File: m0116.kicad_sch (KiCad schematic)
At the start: 256 parts, among them J2 Conn_01x04_MountingPin, J3 Conn_01x04_MountingPin, Q1 Q_PMOS_GSD AO3401A, Q2 Q_NMOS_GSD 2N7002, Q3 Q_NMOS_GSD 2N7002, Q4 2N3904, SW1 SW_Push, U1 XC6206P332MR, U2 74AHCT1G125, U3 STM32F411RETx, U4 24LC64, U5 USBLC6-2SC6, Y1 8MHz

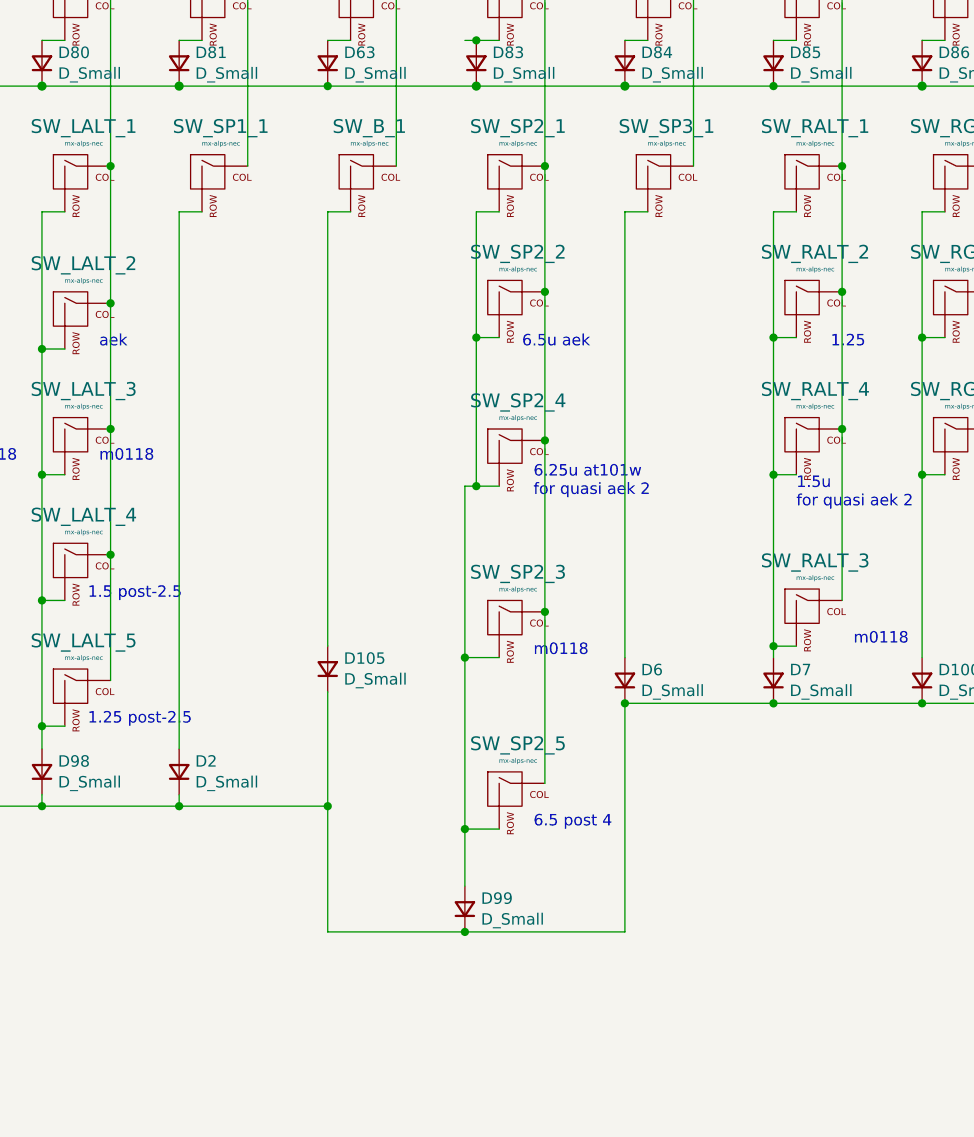
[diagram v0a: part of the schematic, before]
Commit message: fix
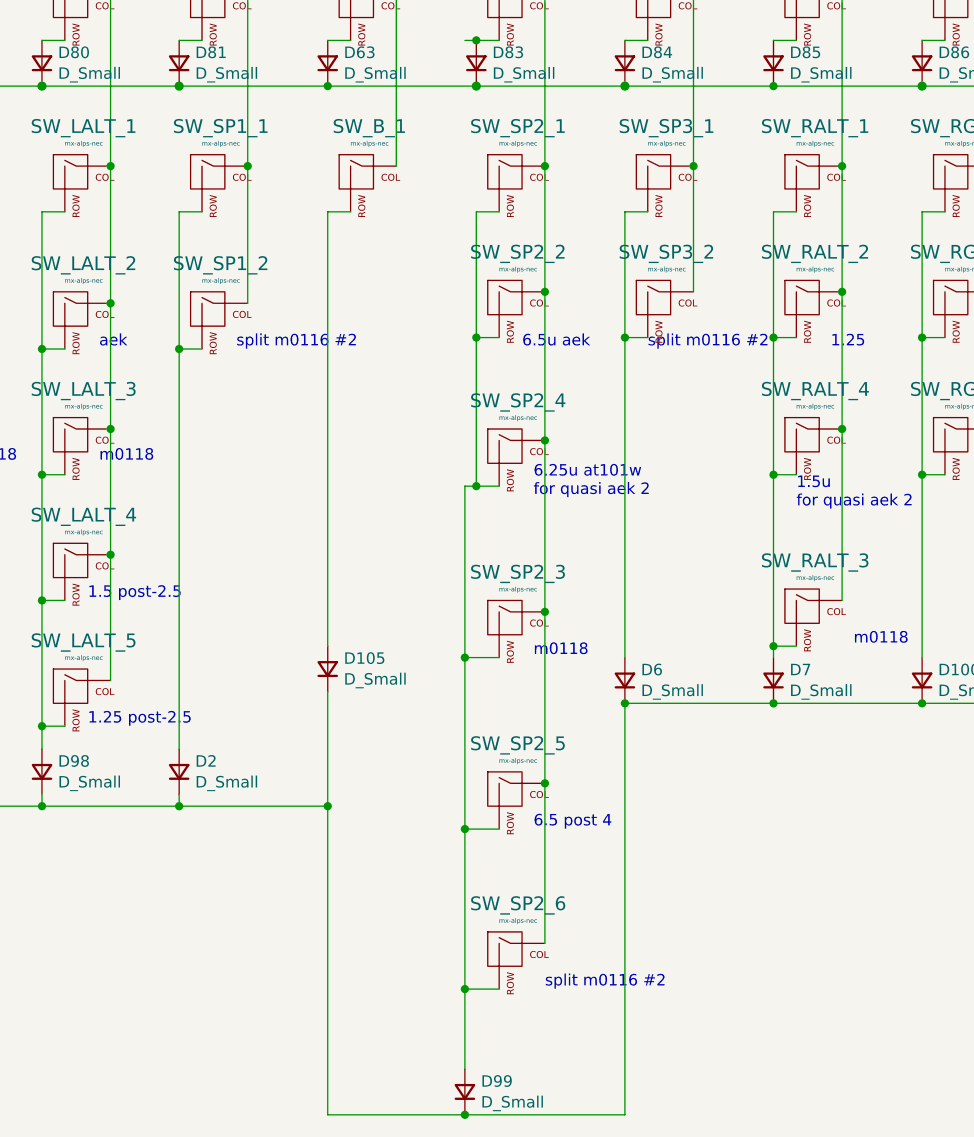
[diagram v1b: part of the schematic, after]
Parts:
- added SW_SP1_2, SW_SP2_6, SW_SP3_2: mx-alps-nec, Alps_Only:ALPS-1U, symbol MX_Alps_Hybrid:mx-alps-nec
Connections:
- net COL4: now also SW_SP1_2.1 (COL)
- net COL6: now also SW_SP2_6.1 (COL)
- net COL7: now also SW_SP3_2.1 (COL)
- net at D2.2 (A), SW_SP1_1.2 (ROW): now also SW_SP1_2.2 (ROW)
- net at D6.2 (A), SW_SP3_1.2 (ROW): now also SW_SP3_2.2 (ROW)
- net at D99.2 (A), SW_SP2_1.2 (ROW), SW_SP2_2.2 (ROW)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: now also SW_SP2_6.2 (ROW)
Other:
- note added: "split m0116 #2"
- moved on the sheet: D99
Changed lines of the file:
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@@
   (junction (at 160.02 377.19) (diameter 0) (color 0 0 0 0)
   )
+  (junction (at 93.98 363.22) (diameter 0) (color 0 0 0 0)
+  )
   (junction (at 204.47 65.405) (diameter 0) (color 0 0 0 0)
   )
@@
   (junction (at 86.36 342.9) (diameter 0) (color 0 0 0 0)
   )
+  (junction (at 151.13 342.9) (diameter 0) (color 0 0 0 0)
+  )
   (junction (at 118.11 266.7) (diameter 0) (color 0 0 0 0)
   )
@@
   (junction (at 257.81 361.95) (diameter 0) (color 0 0 0 0)
   )
-  (junction (at 125.73 427.99) (diameter 0) (color 0 0 0 0)
+  (junction (at 125.73 448.31) (diameter 0) (color 0 0 0 0)
   )
   (junction (at 127 328.93) (diameter 0) (color 0 0 0 0)
@@
   (junction (at 33.02 276.86) (diameter 1.016) (color 0 0 0 0)
   )
+  (junction (at 101.6 342.9) (diameter 0) (color 0 0 0 0)
+  )
   (junction (at 101.6 304.8) (diameter 0) (color 0 0 0 0)
   )
@@
   (junction (at 332.74 118.11) (diameter 0) (color 0 0 0 0)
   )
+  (junction (at 134.62 411.48) (diameter 0) (color 0 0 0 0)
+  )
   (junction (at 55.88 358.14) (diameter 0) (color 0 0 0 0)
   )
@@
   (junction (at 93.98 414.02) (diameter 0) (color 0 0 0 0)
   )
+  (junction (at 125.73 434.34) (diameter 0) (color 0 0 0 0)
+  )
   (junction (at 290.83 276.86) (diameter 1.016) (color 0 0 0 0)
   )
@@
   (junction (at 36.83 35.56) (diameter 0) (color 0 0 0 0)
   )
+  (junction (at 143.51 361.95) (diameter 0) (color 0 0 0 0)
+  )
   (junction (at 217.17 323.85) (diameter 0) (color 0 0 0 0)
   )
@@
     (stroke (width 0) (type solid))
   )
-  (wire (pts (xy 93.98 347.98) (xy 93.98 407.67))
+  (wire (pts (xy 93.98 347.98) (xy 93.98 363.22))
     (stroke (width 0) (type default))
   )
@@
     (stroke (width 0) (type solid))
   )
+  (wire (pts (xy 125.73 434.34) (xy 125.73 416.56))
+    (stroke (width 0) (type default))
+  )
   (wire (pts (xy 118.11 259.08) (xy 118.11 266.7))
     (stroke (width 0) (type default))
@@
     (stroke (width 0) (type default))
   )
-  (wire (pts (xy 110.49 427.99) (xy 110.49 414.02))
+  (wire (pts (xy 110.49 448.31) (xy 110.49 414.02))
     (stroke (width 0) (type default))
   )
@@
     (stroke (width 0) (type default))
   )
+  (wire (pts (xy 125.73 434.34) (xy 129.54 434.34))
+    (stroke (width 0) (type default))
+  )
   (wire (pts (xy 184.785 36.83) (xy 172.72 36.83))
     (stroke (width 0) (type default))
@@
     (stroke (width 0) (type solid))
   )
+  (wire (pts (xy 134.62 411.48) (xy 134.62 429.26))
+    (stroke (width 0) (type default))
+  )
   (wire (pts (xy 49.53 153.67) (xy 49.53 157.48))
     (stroke (width 0) (type default))
@@
     (stroke (width 0) (type solid))
   )
+  (wire (pts (xy 93.98 363.22) (xy 96.52 363.22))
+    (stroke (width 0) (type default))
+  )
   (wire (pts (xy 33.02 271.78) (xy 35.56 271.78))
     (stroke (width 0) (type solid))
@@
     (stroke (width 0) (type default))
   )
-  (wire (pts (xy 143.51 427.99) (xy 143.51 402.59))
+  (wire (pts (xy 143.51 448.31) (xy 143.51 402.59))
     (stroke (width 0) (type default))
   )
@@
     (stroke (width 0) (type default))
   )
+  (wire (pts (xy 143.51 361.95) (xy 143.51 397.51))
+    (stroke (width 0) (type default))
+  )
   (wire (pts (xy 176.53 328.93) (xy 179.07 328.93))
     (stroke (width 0) (type solid))
@@
     (stroke (width 0) (type default))
   )
-  (wire (pts (xy 143.51 347.98) (xy 143.51 397.51))
+  (wire (pts (xy 143.51 347.98) (xy 143.51 361.95))
     (stroke (width 0) (type default))
   )
@@
     (stroke (width 0) (type solid))
   )
-  (wire (pts (xy 110.49 427.99) (xy 125.73 427.99))
+  (wire (pts (xy 110.49 448.31) (xy 125.73 448.31))
     (stroke (width 0) (type default))
   )
@@
     (stroke (width 0) (type solid))
   )
-  (wire (pts (xy 125.73 427.99) (xy 143.51 427.99))
+  (wire (pts (xy 125.73 448.31) (xy 143.51 448.31))
     (stroke (width 0) (type default))
   )
@@
     (stroke (width 0) (type solid))
   )
+  (wire (pts (xy 93.98 363.22) (xy 93.98 407.67))
+    (stroke (width 0) (type default))
+  )
   (wire (pts (xy 85.09 84.455) (xy 87.63 84.455))
     (stroke (width 0) (type default))
@@
     (stroke (width 0) (type default))
   )
+  (wire (pts (xy 143.51 361.95) (xy 146.05 361.95))
+    (stroke (width 0) (type default))
+  )
   (wire (pts (xy 124.46 132.08) (xy 125.73 132.08))
     (stroke (width 0) (type default))
@@
     (stroke (width 0) (type solid))
   )
+  (wire (pts (xy 101.6 342.9) (xy 101.6 358.14))
+    (stroke (width 0) (type default))
+  )
   (wire (pts (xy 55.88 304.8) (xy 55.88 323.85))
     (stroke (width 0) (type solid))
@@
     (stroke (width 0) (type default))
   )
-  (wire (pts (xy 125.73 422.91) (xy 125.73 416.56))
+  (wire (pts (xy 125.73 443.23) (xy 125.73 434.34))
     (stroke (width 0) (type default))
   )
@@
     (stroke (width 0) (type default))
   )
+  (wire (pts (xy 151.13 342.9) (xy 151.13 356.87))
+    (stroke (width 0) (type default))
+  )
   (wire (pts (xy 226.06 381) (xy 242.57 381))
     (stroke (width 0) (type solid))
@@
     (effects (font (size 1.27 1.27)) (justify left bottom))
   )
+  (text "split m0116 #2\n" (at 146.05 363.22 0)
+    (effects (font (size 1.27 1.27)) (justify left bottom))
+  )
   (text "aek\n" (at 53.34 363.22 0)
     (effects (font (size 1.27 1.27)) (justify left bottom))
@@
     (effects (font (size 1.27 1.27)) (justify left bottom))
   )
+  (text "split m0116 #2" (at 100.33 363.22 0)
+    (effects (font (size 1.27 1.27)) (justify left bottom))
+  )
   (text "6.5u aek" (at 132.08 363.22 0)
     (effects (font (size 1.27 1.27)) (justify left bottom))
@@
     (effects (font (size 1.27 1.27)) (justify left bottom))
   )
+  (text "split m0116 #2" (at 134.62 434.34 0)
+    (effects (font (size 1.27 1.27)) (justify left bottom))
+  )
   (text "Has resistor in case this pin accidentally\ngets configured as output and gets pulled up"
     (at 52.07 182.88 0)
@@
     )
   )
-  (symbol (lib_id "Device:D_Small") (at 125.73 425.45 90) (unit 1)
+  (symbol (lib_id "Device:D_Small") (at 125.73 445.77 90) (unit 1)
     (in_bom yes) (on_board yes) (dnp no)
-    (property "Reference" "D99" (at 127.508 424.2816 90)
+    (property "Reference" "D99" (at 127.508 444.6016 90)
       (effects (font (size 1.27 1.27)) (justify right))
     )
-    (property "Value" "D_Small" (at 127.508 426.593 90)
+    (property "Value" "D_Small" (at 127.508 446.913 90)
       (effects (font (size 1.27 1.27)) (justify right))
     )
-    (property "Footprint" "Diode_SMD:D_SOD-123" (at 125.73 425.45 90)
+    (property "Footprint" "Diode_SMD:D_SOD-123" (at 125.73 445.77 90)
       (effects (font (size 1.27 1.27)) hide)
     )
-    (property "Datasheet" "~" (at 125.73 425.45 90)
+    (property "Datasheet" "~" (at 125.73 445.77 90)
       (effects (font (size 1.27 1.27)) hide)
     )
@@
     )
   )
+  (symbol (lib_id "MX_Alps_Hybrid:mx-alps-nec") (at 97.79 359.41 0) (unit 1)
+    (in_bom yes) (on_board yes) (dnp no)
+    (property "Reference" "SW_SP1_2" (at 98.6282 353.7458 0)
+      (effects (font (size 1.524 1.524)))
+    )
+    (property "Value" "mx-alps-nec" (at 98.6282 355.6254 0)
+      (effects (font (size 0.508 0.508)))
+    )
+    (property "Footprint" "Alps_Only:ALPS-1U" (at 81.915 360.045 0)
+      (effects (font (size 1.524 1.524)) hide)
+    )
+    (property "Datasheet" "" (at 81.915 360.045 0)
+      (effects (font (size 1.524 1.524)) hide)
+    )
+    (pin "1")
+    (pin "2")
+    (instances
+      (project "m0116"
+        (path "/151da08b-0979-4785-a9bf-6fa9b165d629"
+          (reference "SW_SP1_2") (unit 1)
+        )
+      )
+    )
+  )
   (symbol (lib_id "Device:C_Small") (at 228.6 118.11 270) (unit 1)
     (in_bom yes) (on_board yes) (dnp no)
@@
     )
   )
+  (symbol (lib_id "MX_Alps_Hybrid:mx-alps-nec") (at 130.81 430.53 0) (unit 1)
+    (in_bom yes) (on_board yes) (dnp no)
+    (property "Reference" "SW_SP2_6" (at 131.6482 424.8658 0)
+      (effects (font (size 1.524 1.524)))
+    )
+    (property "Value" "mx-alps-nec" (at 131.6482 426.7454 0)
+      (effects (font (size 0.508 0.508)))
+    )
+    (property "Footprint" "Alps_Only:ALPS-1U" (at 114.935 431.165 0)
+      (effects (font (size 1.524 1.524)) hide)
+    )
+    (property "Datasheet" "" (at 114.935 431.165 0)
+      (effects (font (size 1.524 1.524)) hide)
+    )
+    (pin "1")
+    (pin "2")
+    (instances
+      (project "m0116"
+        (path "/151da08b-0979-4785-a9bf-6fa9b165d629"
+          (reference "SW_SP2_6") (unit 1)
+        )
+      )
+    )
+  )
   (symbol (lib_id "MX_Alps_Hybrid:mx-alps-nec") (at 82.55 401.32 0) (unit 1)
     (in_bom yes) (on_board yes) (dnp no)
@@
         )
       )
+    )
+  )
+  (symbol (lib_id "MX_Alps_Hybrid:mx-alps-nec") (at 147.32 358.14 0) (unit 1)
+    (in_bom yes) (on_board yes) (dnp no)
+    (property "Reference" "SW_SP3_2" (at 148.1582 352.4758 0)
+      (effects (font (size 1.524 1.524)))
+    )
+    (property "Value" "mx-alps-nec" (at 148.1582 354.3554 0)
+      (effects (font (size 0.508 0.508)))
+    )
+    (property "Footprint" "Alps_Only:ALPS-1U" (at 131.445 358.775 0)
+      (effects (font (size 1.524 1.524)) hide)
+    )
+    (property "Datasheet" "" (at 131.445 358.775 0)
+      (effects (font (size 1.524 1.524)) hide)
+    )
+    (pin "1")
+    (pin "2")
+    (instances
+      (project "m0116"
+        (path "/151da08b-0979-4785-a9bf-6fa9b165d629"
+          (reference "SW_SP3_2") (unit 1)
+        )
+      )
